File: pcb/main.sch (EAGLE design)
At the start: 11 parts

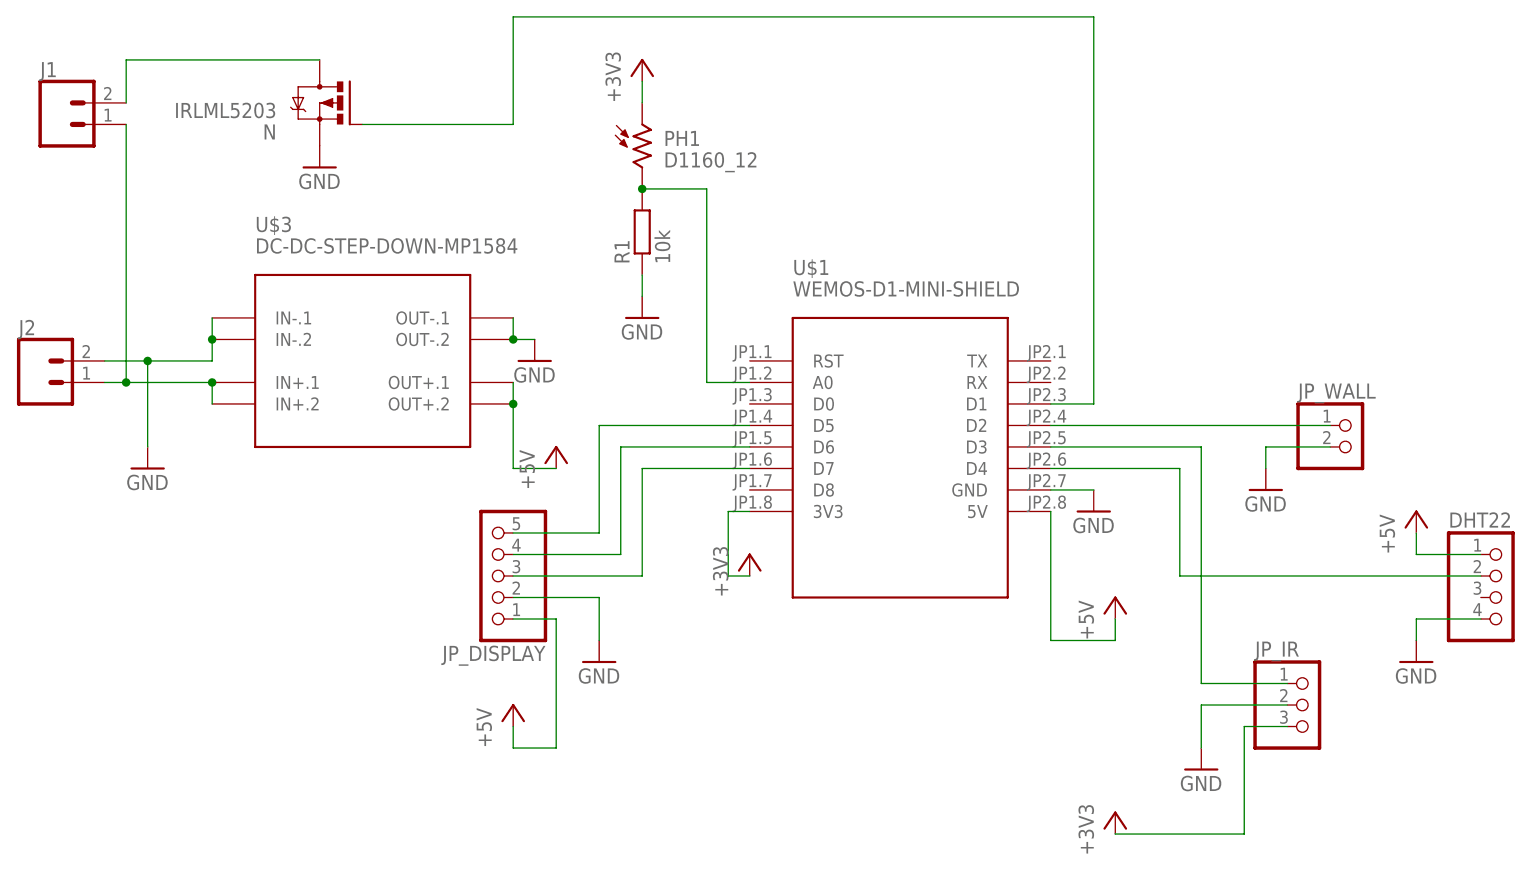
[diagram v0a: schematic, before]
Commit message: upd
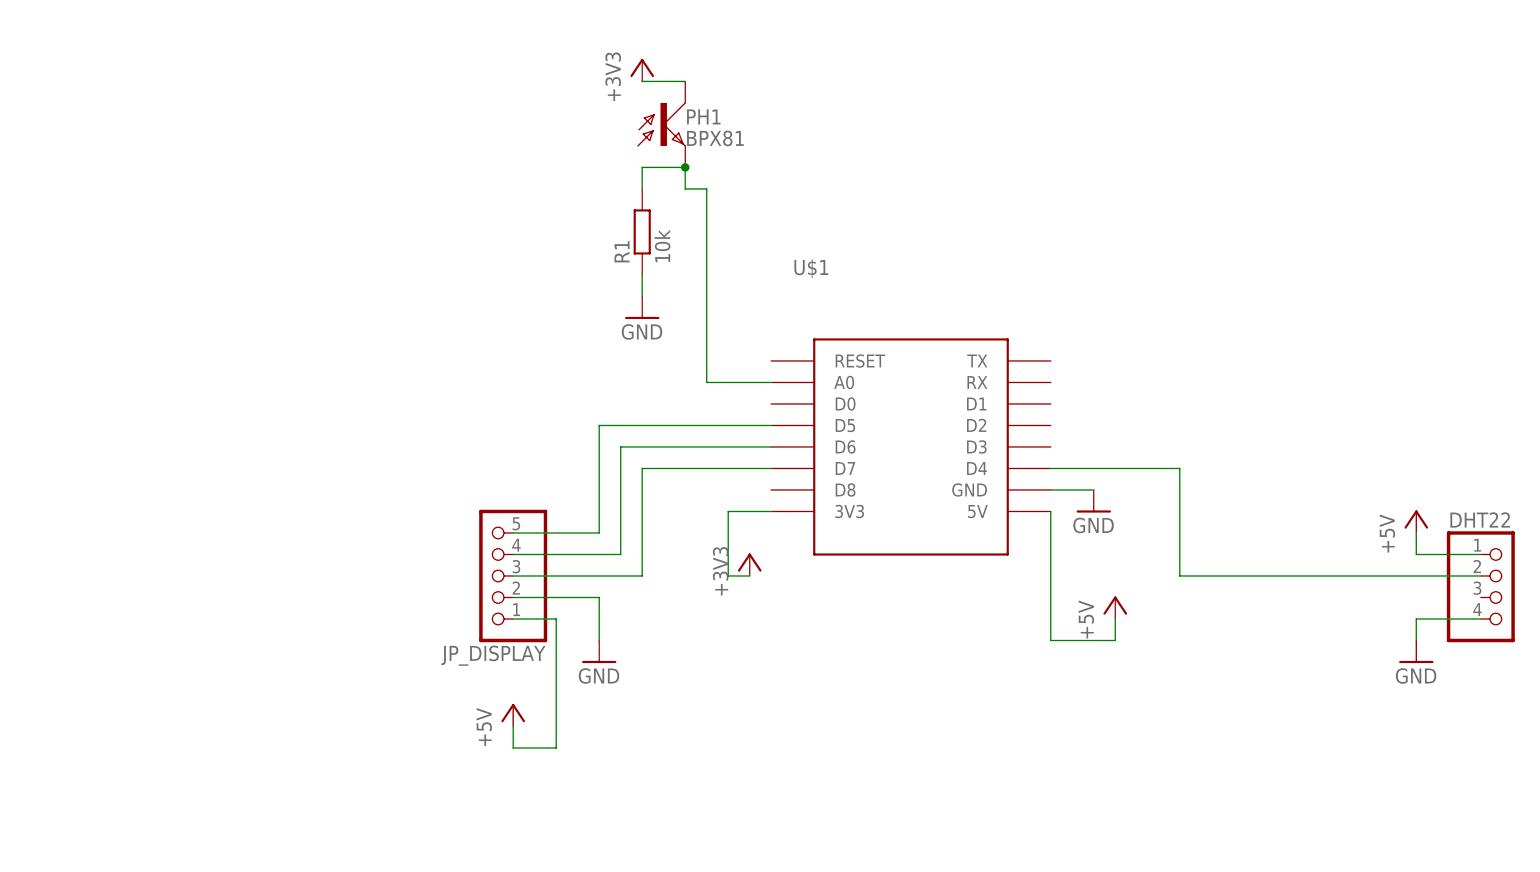
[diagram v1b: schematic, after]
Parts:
- removed J1, J2: (no value), SparkFun-Connectors:CONN_025MM
- removed JP_IR: (no value), pinhead:PINHD-1X3/90
- removed JP_WALL: (no value), pinhead:PINHD-1X2
- removed N: IRLML5203, transistor-power:IRLML5203
- removed U$3: DC-DC-STEP-DOWN-MP1584, diy-modules:DC-DC-STEP-DOWN-MP1584
- PH1: value D1160_12 -> BPX81; device photo-elements:D1160_12 -> opto-trans-siemens:BPX81
- U$1: value WEMOS-D1-MINI-SHIELD -> (none); device diy-modules:WEMOS-D1-MINI-SHIELD -> esp8266modules:WEMOS-D1-MINI
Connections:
- removed net N$1: J1.1, J2.1, U$3.IN+.1, U$3.IN+.2
- removed net N$12: N.G, U$1.D1
- removed net N$3: J1.2, N.D
- removed net N$5: JP_IR.1, U$1.D3
- removed net N$8: JP_WALL.1, U$1.D2
- net +3V3: now also PH1.C; no longer JP_IR.3, PH1.1
- net +5V: no longer U$3.OUT+.1, U$3.OUT+.2
- net GND: no longer J2.2, JP_IR.2, JP_WALL.2, N.S, U$3.IN-.1, U$3.IN-.2, U$3.OUT-.1, U$3.OUT-.2
- net N$2: now also PH1.E; no longer PH1.2
